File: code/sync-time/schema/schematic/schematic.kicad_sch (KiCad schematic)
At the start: 14 parts

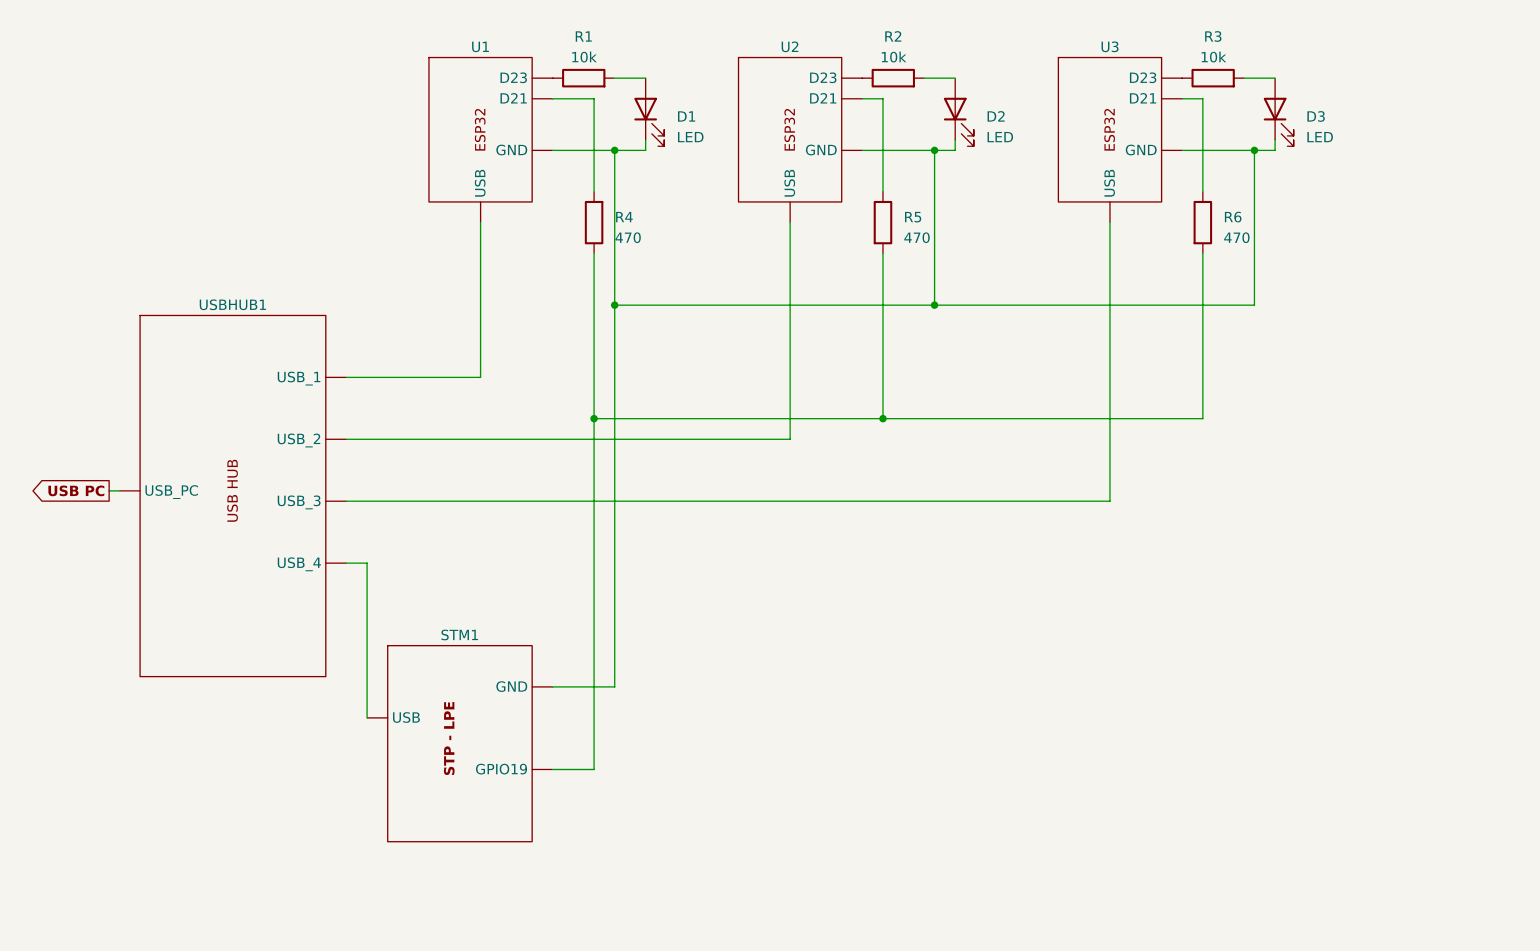
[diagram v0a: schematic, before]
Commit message: Update schema
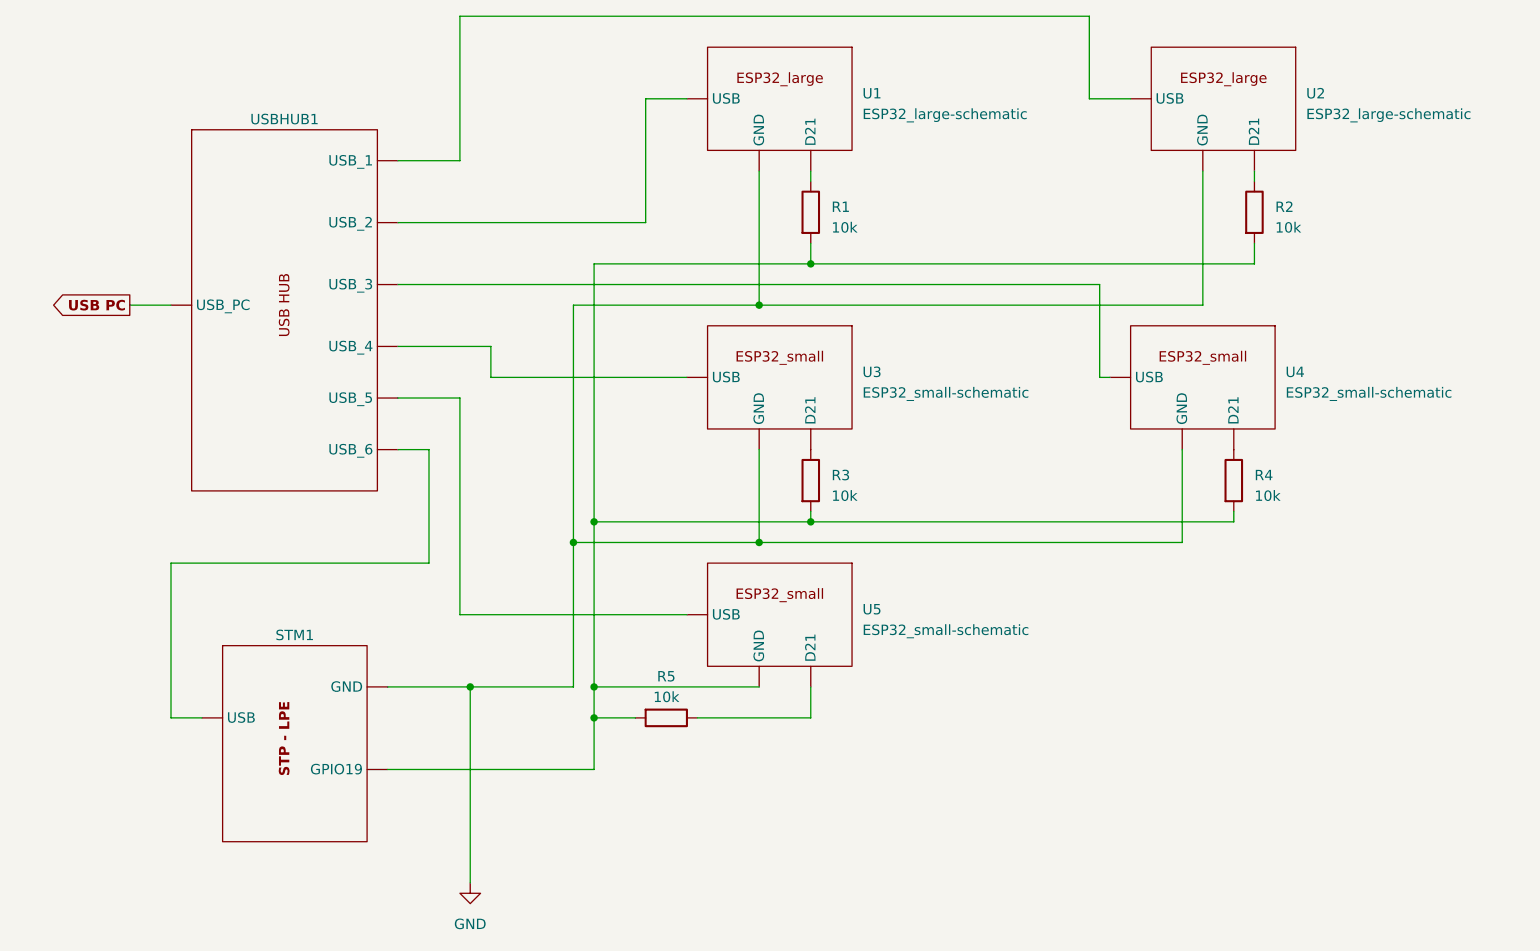
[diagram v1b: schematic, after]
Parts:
- removed D1, D2, D3: LED, symbol Device:LED
- removed R6: 470, symbol Device:R
- removed U1, U2, U3: ~, symbol EspressIf:ESP32-schematic
- added U1, U2: ESP32_large-schematic, symbol EspressIf:ESP32_large-schematic
- added U3, U4, U5: ESP32_small-schematic, symbol EspressIf:ESP32_small-schematic
- R4, R5: value 470 -> 10k
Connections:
- net at R2.1: now also U2. (USB)
- net at R2.2: now also R1.2, R3.2, R4.2, R5.2, STM1. (USB), U5. (USB)
- net GND: now reaches STM1. (USB)
- net GND: now also U1. (USB), U2. (USB), U3. (USB), U4. (USB); no longer USBHUB1. (USB_PC)
- net at R5.1: now also U5. (USB)
- net at R3.1: now also U3. (USB)
- net at R1.1: now also U1. (USB)
- new net: STM1. (USB), USBHUB1. (USB_PC)
- new net: U2. (USB), USBHUB1. (USB_PC)
- new net: U5. (USB), USBHUB1. (USB_PC)
- new net: U1. (USB), USBHUB1. (USB_PC)
- new net: U4. (USB), USBHUB1. (USB_PC)
- new net: U3. (USB), USBHUB1. (USB_PC)
- new net: R4.1, U4. (USB)
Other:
- title: Zapojeni pro mereni vlastnosti protokolu ESP-NOW -> Zapojení pro měření sycnronizace času
- moved on the sheet: STM1

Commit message: Add chapt about sync time
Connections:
- net at U5. (USB): now also R5.1; no longer USBHUB1. (USB_PC)
- new net: STM1. (USB), USBHUB1. (USB_PC)
- new net: U2. (USB), USBHUB1. (USB_PC)
- new net: U5. (USB), USBHUB1. (USB_PC)
- new net: U1. (USB), USBHUB1. (USB_PC)
- new net: U4. (USB), USBHUB1. (USB_PC)
- new net: U3. (USB), USBHUB1. (USB_PC)
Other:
- title: Zapojení pro měření sycnronizace času -> Zapojení pro měření synchronizace času
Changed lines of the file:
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@@
   (paper "A5")
   (title_block
-    (title "Zapojení pro měření sycnronizace času")
+    (title "Zapojení pro měření synchronizace času")
   )
   (junction (at 81.28 80.01) (diameter 0) (color 0 0 0 0)
